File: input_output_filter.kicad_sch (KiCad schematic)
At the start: 36 parts, among them J1 NC3MAH, J10 AudioJack3, J11 AudioJack3, J2 NC3MAH, J3 NC3MAH, J4 NC3MAH, J5 XLR3_AudioJack3_Combo_Ground, J6 XLR3_AudioJack3_Combo_Ground, SW6 SW_SPST, SW7 SW_SPST

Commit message: bom completata
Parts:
- C24, C25, C26, C29, C32, C35: footprint Capacitor_SMD:C_1210_3225Metric -> Capacitor_SMD:C_0805_2012Metric
- J10, J11: footprint Connector_Audio:Jack_3.5mm_Lumberg_1503_07_Horizontal -> Connector_Audio:Jack_3.5mm_CUI_SJ1-3523N_Horizontal

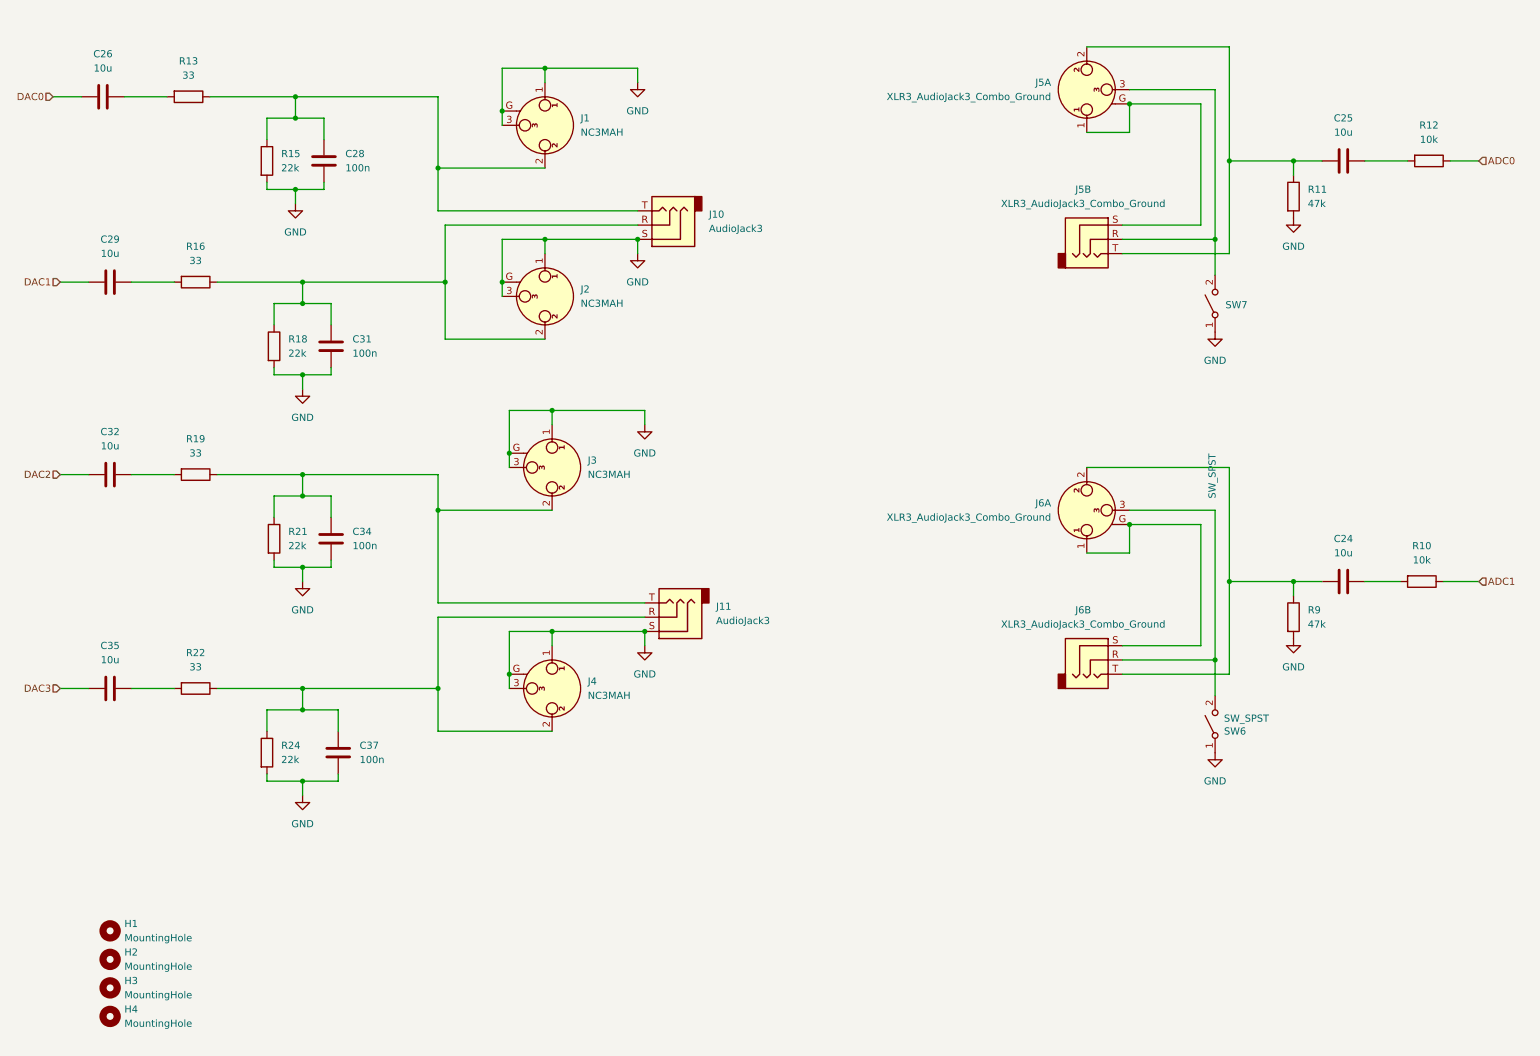
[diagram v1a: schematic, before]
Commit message: pulito lo schematico e fatto dei check
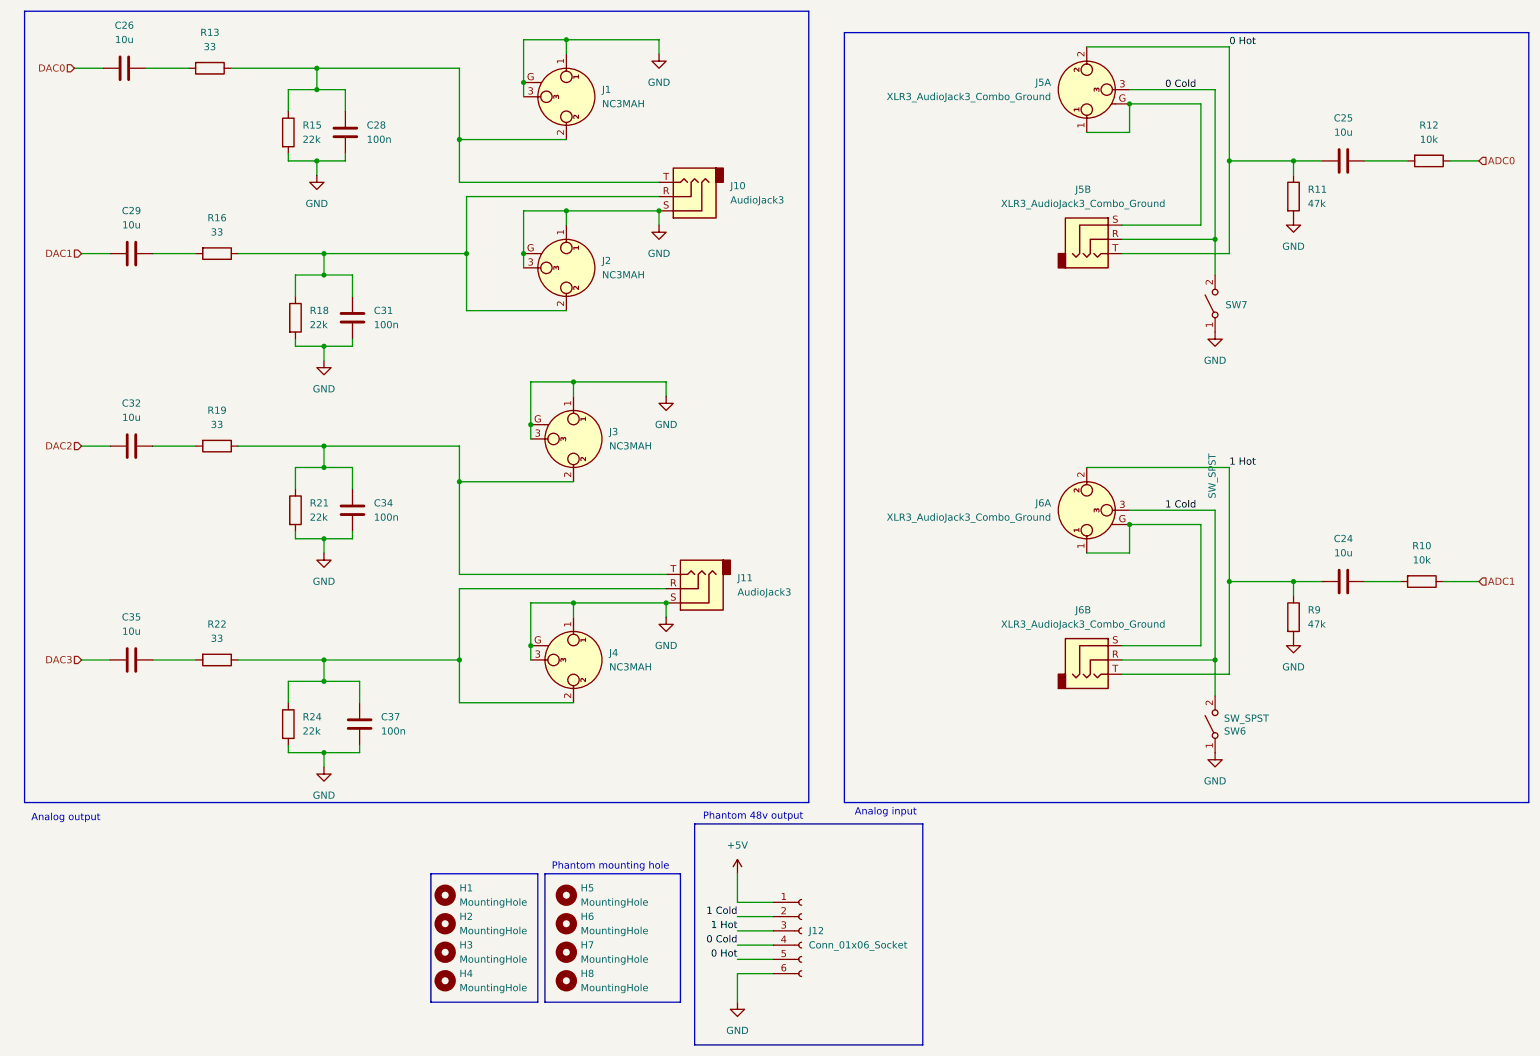
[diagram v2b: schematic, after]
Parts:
- added H5, H6, H7, H8: MountingHole, MountingHole:MountingHole_2.2mm_M2_Pad_Via, symbol Mechanical:MountingHole
- added J12: Conn_01x06_Socket, Connector_PinHeader_2.54mm:PinHeader_1x06_P2.54mm_Vertical, symbol Connector:Conn_01x06_Socket
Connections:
- net GND: now also J12.6 (Pin_6)
- net 1 Hot: now reaches C24.1, J6.2, J6.T, R9.1
- net 1 Hot: now also J12.3 (Pin_3)
- net 1 Cold: now reaches J6.3, J6.R, SW6.2 (B)
- net 1 Cold: now also J12.2 (Pin_2)
- net 0 Hot: now reaches C25.1, J5.2, J5.T, R11.1
- net 0 Hot: now also J12.5 (Pin_5)
- net 0 Cold: now reaches J5.3, J5.R, SW7.2 (B)
- net 0 Cold: now also J12.4 (Pin_4)
- new net +5V: J12.1 (Pin_1)
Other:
- note added: "Analog input"
- note added: "Analog output"
- note added: "Phantom 48v output"
- note added: "Phantom mounting hole"
- moved on the sheet: C26, C28, C29, C31, C32, C34, C35, C37, H1, H2, H3, H4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
